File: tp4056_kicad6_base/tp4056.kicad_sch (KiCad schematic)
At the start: 38 parts, among them J1 Conn_01x01_Female, J2 Conn_01x01_Female, J3 USB_B_Micro, J4 Conn_01x02_Male, J6 Conn_01x05_Male, Q1 AO3401A, Q2 FS8205A, Q3 AO3401A, Q4 AO3401A, Q5 AO3400A, U1 TP4056, U2 DW01, U3 LM1117-3.3, U4 LM809

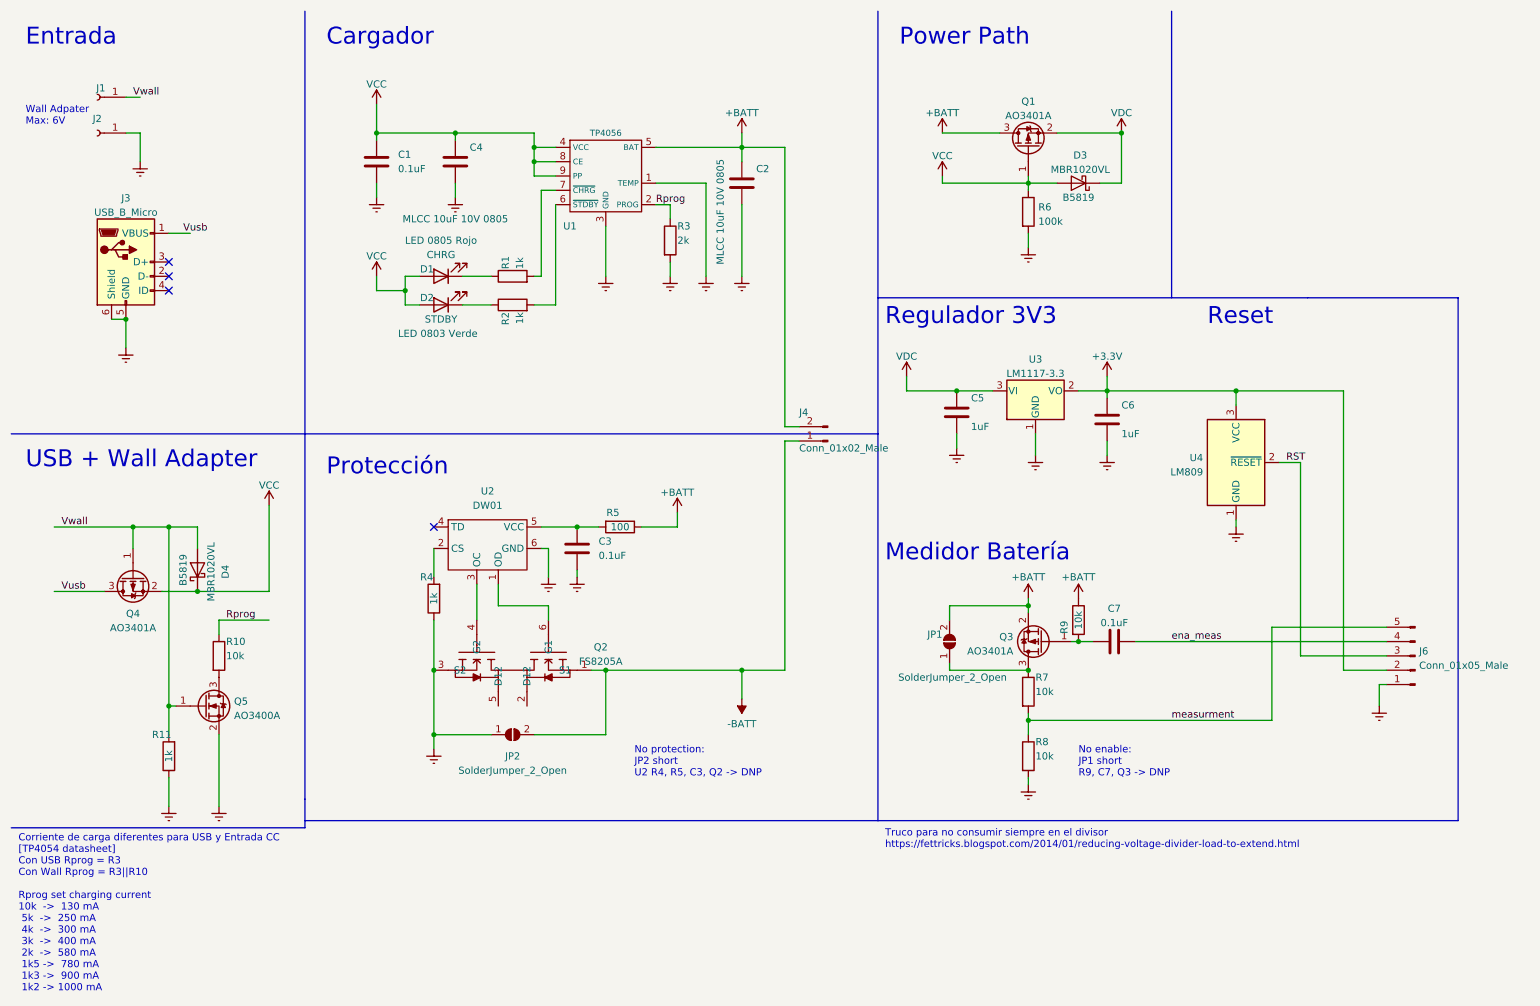
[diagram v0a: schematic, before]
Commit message: PCB. output files. minor cosmetic changes.
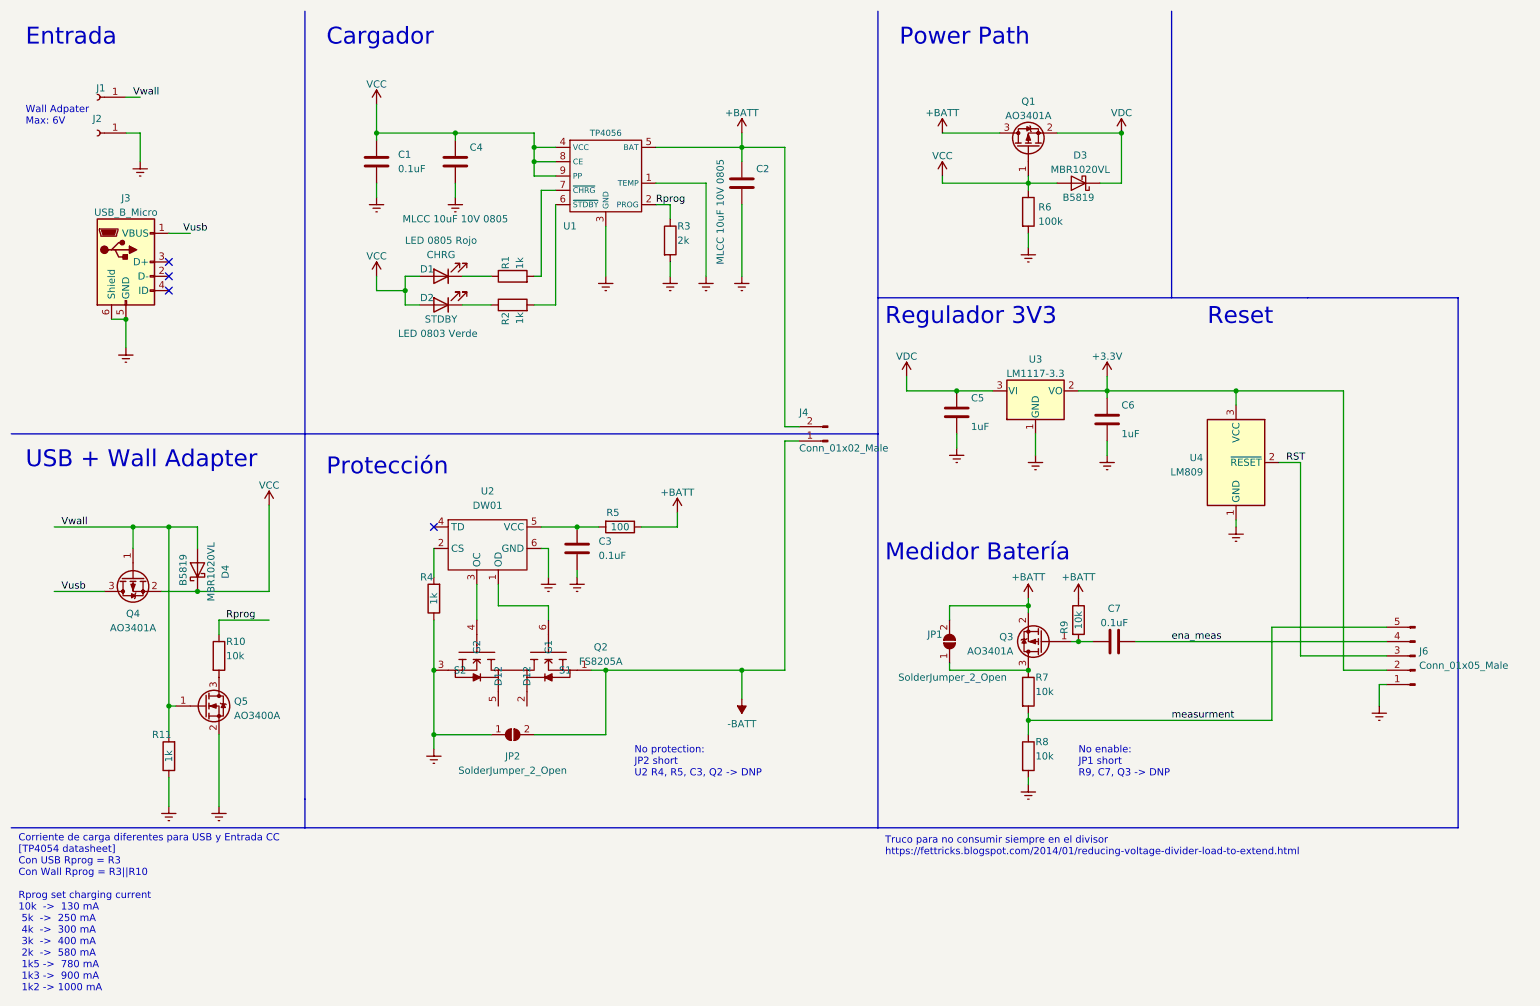
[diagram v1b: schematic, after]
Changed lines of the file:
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@@
     (stroke (width 0) (type default) (color 0 0 0 0))
   )
-  (polyline (pts (xy 267.97 156.21) (xy 267.97 63.5))
+  (polyline (pts (xy 267.97 157.48) (xy 267.97 63.5))
     (stroke (width 0) (type default) (color 0 0 0 0))
   )
@@
     (stroke (width 0) (type default) (color 0 0 0 0))
   )
-  (polyline (pts (xy 165.1 156.21) (xy 267.97 156.21))
+  (polyline (pts (xy 165.1 157.48) (xy 267.97 157.48))
     (stroke (width 0) (type default) (color 0 0 0 0))
   )
@@
     (stroke (width 0) (type default) (color 0 0 0 0))
   )
-  (polyline (pts (xy 165.1 156.21) (xy 165.1 87.63))
+  (polyline (pts (xy 165.1 157.48) (xy 165.1 87.63))
     (stroke (width 0) (type default) (color 0 0 0 0))
   )
@@
     (stroke (width 0) (type default) (color 0 0 0 0))
   )
-  (polyline (pts (xy 63.5 156.21) (xy 165.1 156.21))
+  (polyline (pts (xy 63.5 157.48) (xy 165.1 157.48))
     (stroke (width 0) (type default) (color 0 0 0 0))
   )
@@
   )
   (text "Truco para no consumir siempre en el divisor\nhttps://fettricks.blogspot.com/2014/01/reducing-voltage-divider-load-to-extend.html"
-    (at 166.37 161.29 0)
+    (at 166.37 162.56 0)
     (effects (font (size 1.27 1.27)) (justify left bottom))
   )
